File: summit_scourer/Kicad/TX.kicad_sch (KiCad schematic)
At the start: 10 parts, among them Q1 Q_NMOS, U3 74AC00

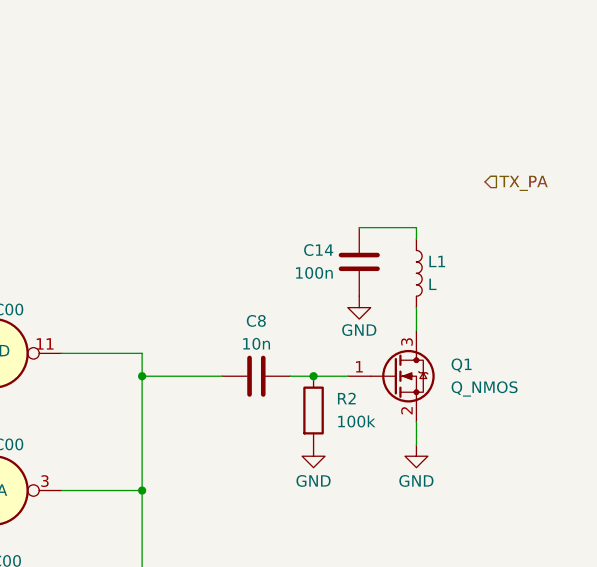
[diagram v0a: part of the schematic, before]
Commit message: Add files via upload
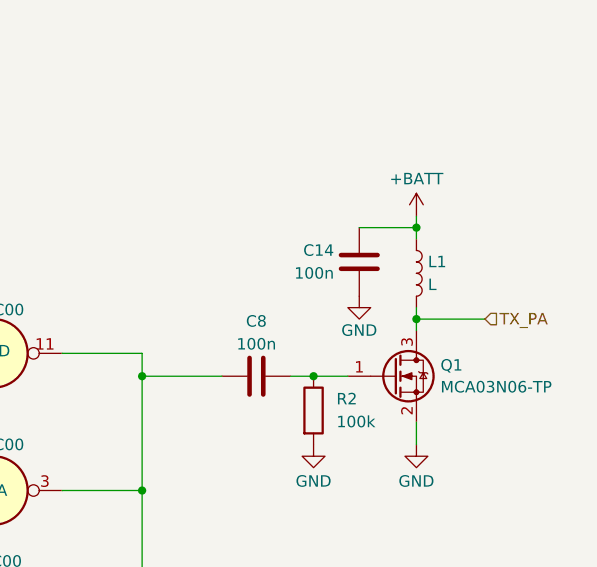
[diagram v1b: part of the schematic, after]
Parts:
- C8: value 10n -> 100n
- Q1: value Q_NMOS -> MCA03N06-TP
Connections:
- net TX_PA: now also L1.2, Q1.3 (D)
- net +BATT: now reaches C14.1, L1.1
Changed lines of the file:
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@@
+	)
+	(junction
+		(at 246.38 123.19)
+		(diameter 0)
+		(color 0 0 0 0)
 	)
 	(junction
@@
 	)
 	(junction
+		(at 246.38 113.03)
+		(diameter 0)
+		(color 0 0 0 0)
+	)
+	(junction
 		(at 153.67 130.81)
 		(diameter 0)
@@
 	(wire
 		(pts
+			(xy 246.38 111.76) (xy 246.38 113.03)
+		)
+		(stroke
+			(width 0)
+			(type default)
+		)
+	)
+	(wire
+		(pts
 			(xy 187.96 124.46) (xy 187.96 133.35)
 		)
@@
 	(wire
 		(pts
-			(xy 246.38 121.92) (xy 246.38 124.46)
+			(xy 246.38 121.92) (xy 246.38 123.19)
 		)
 		(stroke
@@
 	(wire
 		(pts
+			(xy 246.38 123.19) (xy 246.38 124.46)
+		)
+		(stroke
+			(width 0)
+			(type default)
+		)
+	)
+	(wire
+		(pts
 			(xy 190.5 129.54) (xy 190.5 144.78)
 		)
@@
 		(pts
 			(xy 187.96 133.35) (xy 187.96 139.7)
+		)
+		(stroke
+			(width 0)
+			(type default)
+		)
+	)
+	(wire
+		(pts
+			(xy 246.38 123.19) (xy 254 123.19)
 		)
 		(stroke
@@
 	(hierarchical_label "TX_PA"
 		(shape input)
-		(at 254 107.95 0)
+		(at 254 123.19 0)
 		(fields_autoplaced yes)
 		(effects
@@
 		)
 		(instances
-			(project ""
+			(project "summit_scourer"
 				(path "/97fa5a9e-fea2-40ae-976c-23c41ffbf522/ca0b4637-7833-41cb-9c23-66bdf9156fd1"
 					(reference "U3")
@@
 		)
 		(instances
-			(project ""
+			(project "summit_scourer"
 				(path "/97fa5a9e-fea2-40ae-976c-23c41ffbf522/ca0b4637-7833-41cb-9c23-66bdf9156fd1"
 					(reference "L1")
+					(unit 1)
+				)
+			)
+		)
+	)
+	(symbol
+		(lib_id "power:+BATT")
+		(at 246.38 111.76 0)
+		(unit 1)
+		(exclude_from_sim no)
+		(in_bom yes)
+		(on_board yes)
+		(dnp no)
+		(fields_autoplaced yes)
+		(property "Reference" "#PWR023"
+			(at 246.38 115.57 0)
+			(effects
+				(font
+					(size 1.27 1.27)
+				)
+				(hide yes)
+			)
+		)
+		(property "Value" "+BATT"
+			(at 246.38 107.6269 0)
+			(effects
+				(font
+					(size 1.27 1.27)
+				)
+			)
+		)
+		(property "Footprint" ""
+			(at 246.38 111.76 0)
+			(effects
+				(font
+					(size 1.27 1.27)
+				)
+				(hide yes)
+			)
+		)
+		(property "Datasheet" ""
+			(at 246.38 111.76 0)
+			(effects
+				(font
+					(size 1.27 1.27)
+				)
+				(hide yes)
+			)
+		)
+		(property "Description" "Power symbol creates a global label with name \"+BATT\""
+			(at 246.38 111.76 0)
+			(effects
+				(font
+					(size 1.27 1.27)
+				)
+				(hide yes)
+			)
+		)
+		(pin "1"
+		)
+		(instances
+			(project "summit_scourer"
+				(path "/97fa5a9e-fea2-40ae-976c-23c41ffbf522/ca0b4637-7833-41cb-9c23-66bdf9156fd1"
+					(reference "#PWR023")
 					(unit 1)
 				)
@@
 		)
 		(instances
-			(project ""
+			(project "summit_scourer"
 				(path "/97fa5a9e-fea2-40ae-976c-23c41ffbf522/ca0b4637-7833-41cb-9c23-66bdf9156fd1"
 					(reference "U3")
@@
 			)
 		)
-		(property "Value" "10n"
+		(property "Value" "100n"
 			(at 228.6 125.984 90)
 			(effects
@@
 		)
 		(instances
-			(project ""
+			(project "summit_scourer"
 				(path "/97fa5a9e-fea2-40ae-976c-23c41ffbf522/ca0b4637-7833-41cb-9c23-66bdf9156fd1"
 					(reference "U3")
@@
 		(fields_autoplaced yes)
 		(property "Reference" "Q1"
-			(at 250.19 128.2699 0)
+			(at 249.047 128.3278 0)
 			(effects
 				(font
@@
 			)
 		)
-		(property "Value" "Q_NMOS"
-			(at 250.19 130.8099 0)
+		(property "Value" "MCA03N06-TP"
+			(at 249.047 130.7521 0)
 			(effects
 				(font
@@
 		)
 		(instances
-			(project ""
+			(project "summit_scourer"
 				(path "/97fa5a9e-fea2-40ae-976c-23c41ffbf522/ca0b4637-7833-41cb-9c23-66bdf9156fd1"
 					(reference "Q1")
@@
 		)
 		(instances
-			(project ""
+			(project "summit_scourer"
 				(path "/97fa5a9e-fea2-40ae-976c-23c41ffbf522/ca0b4637-7833-41cb-9c23-66bdf9156fd1"
 					(reference "U3")
@@
 		)
 		(instances
-			(project ""
+			(project "summit_scourer"
 				(path "/97fa5a9e-fea2-40ae-976c-23c41ffbf522/ca0b4637-7833-41cb-9c23-66bdf9156fd1"
 					(reference "R1")
@@
 		)
 		(instances
-			(project ""
+			(project "summit_scourer"
 				(path "/97fa5a9e-fea2-40ae-976c-23c41ffbf522/ca0b4637-7833-41cb-9c23-66bdf9156fd1"
 					(reference "U3")

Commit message: Add files via upload
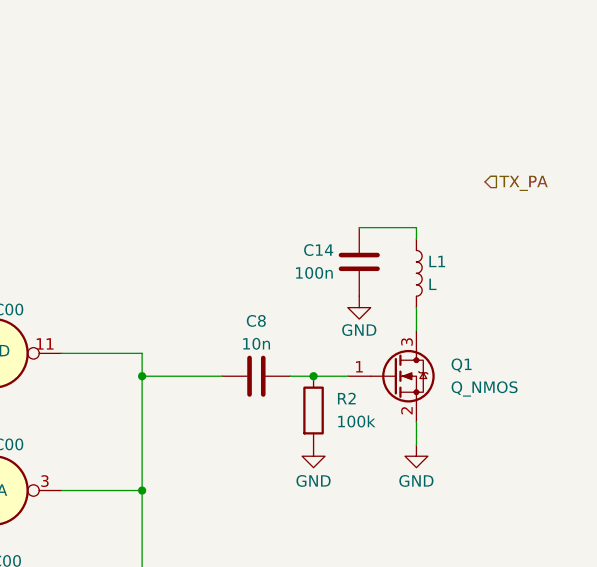
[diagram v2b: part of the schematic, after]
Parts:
- C8: value 100n -> 10n
- Q1: value MCA03N06-TP -> Q_NMOS
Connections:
- net TX_PA: no longer L1.2, Q1.3 (D)
- net +BATT: no longer names the net of C14.1, L1.1
- new net: L1.2, Q1.3 (D)
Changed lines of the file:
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@@
-	)
-	(junction
-		(at 246.38 123.19)
-		(diameter 0)
-		(color 0 0 0 0)
 	)
 	(junction
@@
 	)
 	(junction
-		(at 246.38 113.03)
-		(diameter 0)
-		(color 0 0 0 0)
-	)
-	(junction
 		(at 153.67 130.81)
 		(diameter 0)
@@
 	(wire
 		(pts
-			(xy 246.38 111.76) (xy 246.38 113.03)
-		)
-		(stroke
-			(width 0)
-			(type default)
-		)
-	)
-	(wire
-		(pts
 			(xy 187.96 124.46) (xy 187.96 133.35)
 		)
@@
 	(wire
 		(pts
-			(xy 246.38 121.92) (xy 246.38 123.19)
+			(xy 246.38 121.92) (xy 246.38 124.46)
 		)
 		(stroke
@@
 	(wire
 		(pts
-			(xy 246.38 123.19) (xy 246.38 124.46)
-		)
-		(stroke
-			(width 0)
-			(type default)
-		)
-	)
-	(wire
-		(pts
 			(xy 190.5 129.54) (xy 190.5 144.78)
 		)
@@
 		(pts
 			(xy 187.96 133.35) (xy 187.96 139.7)
-		)
-		(stroke
-			(width 0)
-			(type default)
-		)
-	)
-	(wire
-		(pts
-			(xy 246.38 123.19) (xy 254 123.19)
 		)
 		(stroke
@@
 	(hierarchical_label "TX_PA"
 		(shape input)
-		(at 254 123.19 0)
+		(at 254 107.95 0)
 		(fields_autoplaced yes)
 		(effects
@@
 		)
 		(instances
-			(project "summit_scourer"
+			(project ""
 				(path "/97fa5a9e-fea2-40ae-976c-23c41ffbf522/ca0b4637-7833-41cb-9c23-66bdf9156fd1"
 					(reference "U3")
@@
 		)
 		(instances
-			(project "summit_scourer"
+			(project ""
 				(path "/97fa5a9e-fea2-40ae-976c-23c41ffbf522/ca0b4637-7833-41cb-9c23-66bdf9156fd1"
 					(reference "L1")
-					(unit 1)
-				)
-			)
-		)
-	)
-	(symbol
-		(lib_id "power:+BATT")
-		(at 246.38 111.76 0)
-		(unit 1)
-		(exclude_from_sim no)
-		(in_bom yes)
-		(on_board yes)
-		(dnp no)
-		(fields_autoplaced yes)
-		(property "Reference" "#PWR023"
-			(at 246.38 115.57 0)
-			(effects
-				(font
-					(size 1.27 1.27)
-				)
-				(hide yes)
-			)
-		)
-		(property "Value" "+BATT"
-			(at 246.38 107.6269 0)
-			(effects
-				(font
-					(size 1.27 1.27)
-				)
-			)
-		)
-		(property "Footprint" ""
-			(at 246.38 111.76 0)
-			(effects
-				(font
-					(size 1.27 1.27)
-				)
-				(hide yes)
-			)
-		)
-		(property "Datasheet" ""
-			(at 246.38 111.76 0)
-			(effects
-				(font
-					(size 1.27 1.27)
-				)
-				(hide yes)
-			)
-		)
-		(property "Description" "Power symbol creates a global label with name \"+BATT\""
-			(at 246.38 111.76 0)
-			(effects
-				(font
-					(size 1.27 1.27)
-				)
-				(hide yes)
-			)
-		)
-		(pin "1"
-		)
-		(instances
-			(project "summit_scourer"
-				(path "/97fa5a9e-fea2-40ae-976c-23c41ffbf522/ca0b4637-7833-41cb-9c23-66bdf9156fd1"
-					(reference "#PWR023")
 					(unit 1)
 				)
@@
 		)
 		(instances
-			(project "summit_scourer"
+			(project ""
 				(path "/97fa5a9e-fea2-40ae-976c-23c41ffbf522/ca0b4637-7833-41cb-9c23-66bdf9156fd1"
 					(reference "U3")
@@
 			)
 		)
-		(property "Value" "100n"
+		(property "Value" "10n"
 			(at 228.6 125.984 90)
 			(effects
@@
 		)
 		(instances
-			(project "summit_scourer"
+			(project ""
 				(path "/97fa5a9e-fea2-40ae-976c-23c41ffbf522/ca0b4637-7833-41cb-9c23-66bdf9156fd1"
 					(reference "U3")
@@
 		(fields_autoplaced yes)
 		(property "Reference" "Q1"
-			(at 249.047 128.3278 0)
+			(at 250.19 128.2699 0)
 			(effects
 				(font
@@
 			)
 		)
-		(property "Value" "MCA03N06-TP"
-			(at 249.047 130.7521 0)
+		(property "Value" "Q_NMOS"
+			(at 250.19 130.8099 0)
 			(effects
 				(font
@@
 		)
 		(instances
-			(project "summit_scourer"
+			(project ""
 				(path "/97fa5a9e-fea2-40ae-976c-23c41ffbf522/ca0b4637-7833-41cb-9c23-66bdf9156fd1"
 					(reference "Q1")
@@
 		)
 		(instances
-			(project "summit_scourer"
+			(project ""
 				(path "/97fa5a9e-fea2-40ae-976c-23c41ffbf522/ca0b4637-7833-41cb-9c23-66bdf9156fd1"
 					(reference "U3")
@@
 		)
 		(instances
-			(project "summit_scourer"
+			(project ""
 				(path "/97fa5a9e-fea2-40ae-976c-23c41ffbf522/ca0b4637-7833-41cb-9c23-66bdf9156fd1"
 					(reference "R1")
@@
 		)
 		(instances
-			(project "summit_scourer"
+			(project ""
 				(path "/97fa5a9e-fea2-40ae-976c-23c41ffbf522/ca0b4637-7833-41cb-9c23-66bdf9156fd1"
 					(reference "U3")
